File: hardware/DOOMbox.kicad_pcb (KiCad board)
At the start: 4 copper layers, 84 parts, among them J1 DE15_Socket_HighDensity, J2 AudioJack3, SW1 SW_SPST, SW2 SW_Push, U1 RPi Pico 2, U3 AP7381-50SA-7, U4 LM324N, U5 CD4010BE

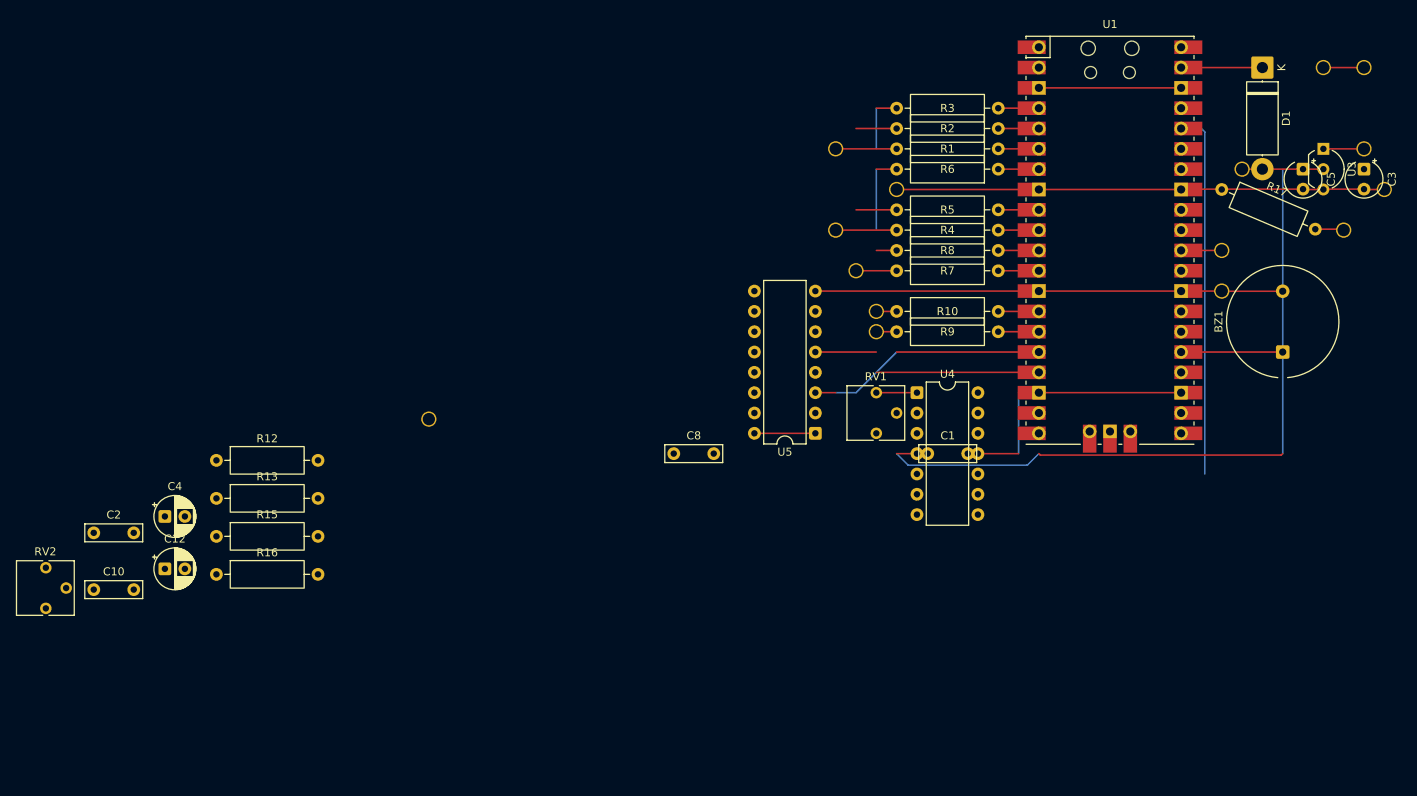
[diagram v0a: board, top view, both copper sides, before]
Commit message: Complete stripboard design
Squashed commit of the following:

commit dbad1e7bdfb2dba54c7140f3a2191c6905e5781a
Author: Jack Bennett <jackbennett0708@gmail.com>
Date:   Sat Aug 30 16:36:03 2025 +0100

    Complete

commit 05059f46a42e6744a15d06e69ba94dfb8af3ae9c
Author: Jack Bennett <jackbennett0708@gmail.com>
Date:   Sat Aug 30 14:41:32 2025 +0100

    1
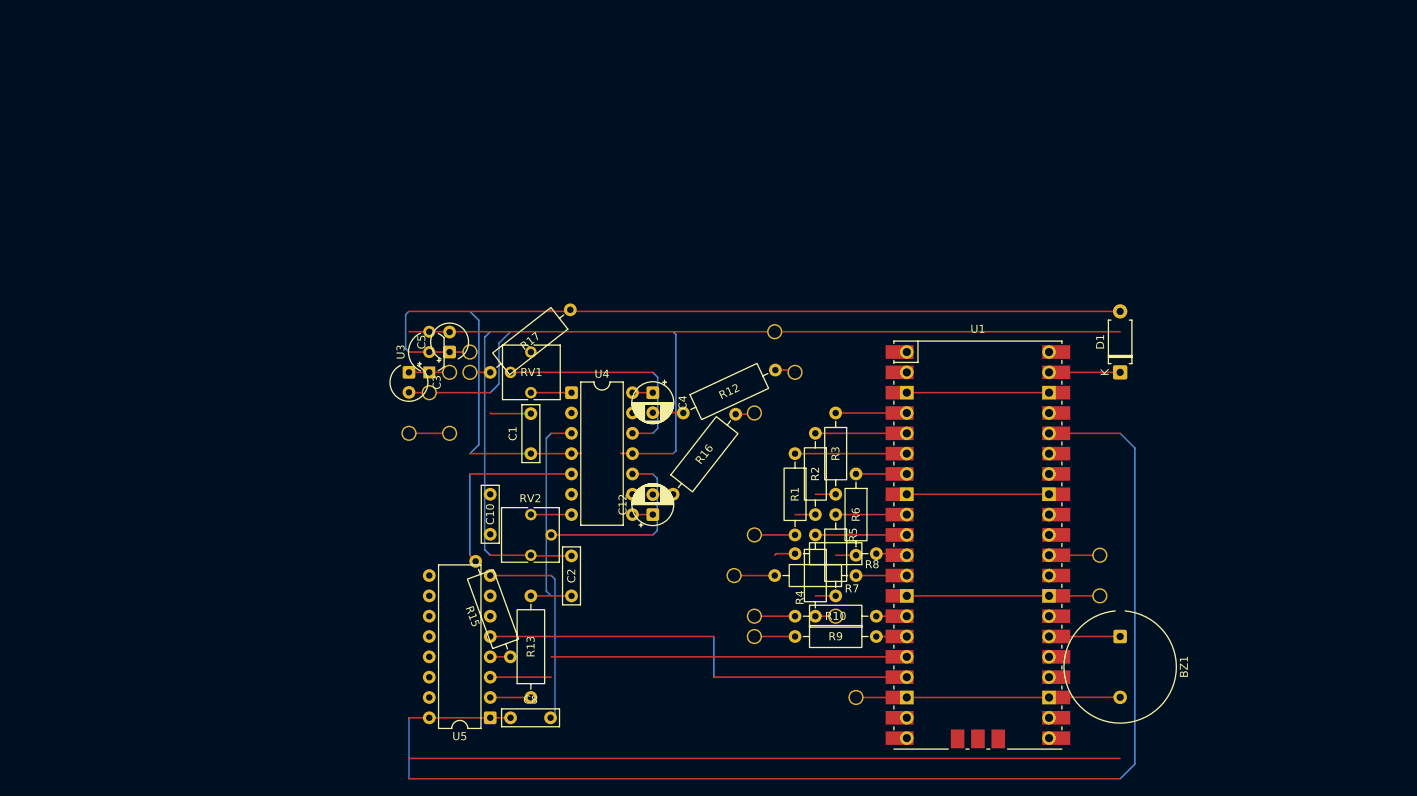
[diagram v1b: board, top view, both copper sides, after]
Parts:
- removed the D2 at (198.1, 48.3)
- removed the D2 at (185.4, 40.6)
- removed the J1 at (139.7, 61.0)
- removed the J1 at (134.6, 48.3)
- removed the J1 at (134.6, 38.1)
- removed the J1 at (142.2, 43.2)
- removed the J1 at (139.7, 58.4)
- removed the J1 at (137.2, 53.3)
- removed the J2 at (83.8, 71.9)
- removed the REF** at (152.4, 40.6)
- removed the REF** at (170.2, 71.1)
- removed the REF** at (141.1, 63.5)
- removed the REF** at (153.8, 71.1)
- removed the REF** at (175.3, 40.6)
- removed the REF** at (175.3, 28.0)
- removed the REF** at (175.3, 50.8)
- removed the REF** at (167.6, 71.1)
- removed the REF** at (193.0, 27.9)
- removed the REF** at (182.9, 40.6)
- removed the REF** at (175.3, 33.0)
- removed the REF** at (152.4, 35.6)
- removed the REF** at (175.3, 35.6)
- removed the REF** at (175.3, 73.7)
- removed the REF** at (198.1, 40.6)
- removed the REF** at (175.3, 63.5)
- removed the REF** at (152.4, 33.0)
- removed the REF** at (203.2, 43.2)
- removed the REF** at (180.3, 25.4)
- removed the REF** at (175.3, 25.4)
- removed the REF** at (175.3, 66.0)
- removed the REF** at (193.0, 48.3)
- removed the REF** at (175.3, 53.3)
- removed the REF** at (175.3, 61.0)
- removed the REF** at (152.4, 50.8)
- removed the REF** at (152.4, 58.4)
- removed the REF** at (175.3, 58.4)
- removed the REF** at (175.3, 38.1)
- removed the REF** at (152.4, 53.3)
- removed the REF** at (175.3, 45.7)
- removed the REF** at (152.4, 48.3)
- removed the REF** at (152.4, 61.0)
- removed the REF** at (180.3, 33.0)
- removed the REF** at (152.4, 45.7)
- removed the REF** at (193.0, 38.1)
- removed the REF** at (175.3, 48.3)
- removed the REF** at (148.6, 76.2)
- removed the REF** at (152.4, 38.1)
- removed the REF** at (175.3, 71.1)
- removed the REF** at (200.7, 27.9)
- removed the SW1 at (200.7, 38.1)
- removed the SW1 at (195.6, 27.9)
- removed the SW2 at (182.9, 50.8)
- removed the SW2 at (182.9, 55.9)
- added ?: , , F.Cu at (124.5, 96.5)
- added ?: , , F.Cu at (134.6, 96.5)
- added ?: , , F.Cu at (124.5, 99.1)
- added ?: , , F.Cu at (137.2, 106.7)
- added ?: , , F.Cu at (121.9, 91.4)
- added D2: LED, Stripboard:Peripheral_Offboard, F.Cu at (88.9, 66.0)
- added J1: DE15_Socket_HighDensity, Stripboard:Peripheral_Offboard, F.Cu at (124.5, 86.4)
- added J2: AudioJack3, Stripboard:Peripheral_Offboard, F.Cu at (127.0, 61.0)
- added J2: AudioJack3, Stripboard:Peripheral_Offboard, F.Cu at (124.5, 71.1)
- added J2: AudioJack3, Stripboard:Peripheral_Offboard, F.Cu at (129.5, 66.0)
- added REF**: Peripheral_Offboard, Stripboard:Peripheral_Offboard, F.Cu at (88.9, 63.5)
- added REF**: Stripboard_Cut, Stripboard:Stripboard_Cut, F.Cu at (126.1, 88.9)
- added REF**: Stripboard_Cut, Stripboard:Stripboard_Cut, F.Cu at (104.1, 83.8)
- added REF**: Stripboard_Cut, Stripboard:Stripboard_Cut, F.Cu at (121.9, 99.1)
- added REF**: Stripboard_Cut, Stripboard:Stripboard_Cut, F.Cu at (154.9, 76.2)
- added REF**: Stripboard_Cut, Stripboard:Stripboard_Cut, F.Cu at (154.9, 99.1)
- added REF**: Stripboard_Cut, Stripboard:Stripboard_Cut, F.Cu at (138.0, 99.0)
- added REF**: Stripboard_Cut, Stripboard:Stripboard_Cut, F.Cu at (154.9, 104.1)
- added REF**: Peripheral_Offboard, Stripboard:Peripheral_Offboard, F.Cu at (81.3, 73.7)
- added REF**: Stripboard_Cut, Stripboard:Stripboard_Cut, F.Cu at (114.3, 83.8)
- added REF**: Stripboard_Cut, Stripboard:Stripboard_Cut, F.Cu at (154.9, 86.4)
- added REF**: Stripboard_Cut, Stripboard:Stripboard_Cut, F.Cu at (131.1, 81.3)
- added REF**: Stripboard_Cut, Stripboard:Stripboard_Cut, F.Cu at (114.3, 68.6)
- added REF**: Stripboard_Cut, Stripboard:Stripboard_Cut, F.Cu at (133.4, 83.8)
- added REF**: Stripboard_Cut, Stripboard:Stripboard_Cut, F.Cu at (104.1, 78.7)
- added REF**: Stripboard_Cut, Stripboard:Stripboard_Cut, F.Cu at (154.9, 109.2)
- added REF**: Stripboard_Cut, Stripboard:Stripboard_Cut, F.Cu at (154.9, 71.1)
- added REF**: Stripboard_Cut, Stripboard:Stripboard_Cut, F.Cu at (110.5, 71.1)
- added REF**: Stripboard_Cut, Stripboard:Stripboard_Cut, F.Cu at (116.8, 81.3)
- added REF**: Stripboard_Cut, Stripboard:Stripboard_Cut, F.Cu at (87.6, 91.4)
- added REF**: Stripboard_Cut, Stripboard:Stripboard_Cut, F.Cu at (119.4, 91.4)
- added REF**: Stripboard_Cut, Stripboard:Stripboard_Cut, F.Cu at (154.9, 96.5)
- added REF**: Stripboard_Cut, Stripboard:Stripboard_Cut, F.Cu at (93.0, 86.3)
- added REF**: Stripboard_Cut, Stripboard:Stripboard_Cut, F.Cu at (129.5, 94.0)
- added REF**: Stripboard_Cut, Stripboard:Stripboard_Cut, F.Cu at (87.6, 106.7)
- added REF**: Stripboard_Cut, Stripboard:Stripboard_Cut, F.Cu at (87.6, 101.6)
- added REF**: Stripboard_Cut, Stripboard:Stripboard_Cut, F.Cu at (114.3, 73.7)
- added REF**: Stripboard_Cut, Stripboard:Stripboard_Cut, F.Cu at (130.7, 86.4)
- added REF**: Stripboard_Cut, Stripboard:Stripboard_Cut, F.Cu at (121.9, 86.4)
- added REF**: Stripboard_Cut, Stripboard:Stripboard_Cut, F.Cu at (133.5, 88.9)
- added REF**: Stripboard_Cut, Stripboard:Stripboard_Cut, F.Cu at (94.0, 63.5)
- added REF**: Stripboard_Cut, Stripboard:Stripboard_Cut, F.Cu at (92.9, 66.1)
- added REF**: Stripboard_Cut, Stripboard:Stripboard_Cut, F.Cu at (110.8, 81.3)
- added REF**: Stripboard_Cut, Stripboard:Stripboard_Cut, F.Cu at (132.1, 91.4)
- added REF**: Stripboard_Cut, Stripboard:Stripboard_Cut, F.Cu at (114.3, 78.7)
- added REF**: Stripboard_Cut, Stripboard:Stripboard_Cut, F.Cu at (154.9, 63.5)
- added REF**: Stripboard_Cut, Stripboard:Stripboard_Cut, F.Cu at (87.6, 94.0)
- added REF**: Stripboard_Cut, Stripboard:Stripboard_Cut, F.Cu at (132.1, 66.0)
- added REF**: Stripboard_Cut, Stripboard:Stripboard_Cut, F.Cu at (121.9, 96.5)
- added REF**: Stripboard_Cut, Stripboard:Stripboard_Cut, F.Cu at (104.1, 71.1)
- added REF**: Stripboard_Cut, Stripboard:Stripboard_Cut, F.Cu at (116.8, 71.1)
- added REF**: Stripboard_Cut, Stripboard:Stripboard_Cut, F.Cu at (149.9, 63.5)
- added REF**: Stripboard_Cut, Stripboard:Stripboard_Cut, F.Cu at (138.0, 96.5)
- added REF**: Stripboard_Cut, Stripboard:Stripboard_Cut, F.Cu at (88.9, 73.7)
- added REF**: Stripboard_Cut, Stripboard:Stripboard_Cut, F.Cu at (87.6, 96.5)
- added REF**: Stripboard_Cut, Stripboard:Stripboard_Cut, F.Cu at (137.2, 94.0)
- added REF**: Stripboard_Cut, Stripboard:Stripboard_Cut, F.Cu at (87.6, 99.1)
- added REF**: Stripboard_Cut, Stripboard:Stripboard_Cut, F.Cu at (154.9, 88.9)
- added REF**: Stripboard_Cut, Stripboard:Stripboard_Cut, F.Cu at (116.8, 76.2)
- added REF**: Stripboard_Cut, Stripboard:Stripboard_Cut, F.Cu at (101.6, 104.1)
- added REF**: Stripboard_Cut, Stripboard:Stripboard_Cut, F.Cu at (128.4, 83.9)
- added REF**: Stripboard_Cut, Stripboard:Stripboard_Cut, F.Cu at (154.9, 101.6)
- added REF**: Stripboard_Cut, Stripboard:Stripboard_Cut, F.Cu at (100.0, 71.0)
- added REF**: Stripboard_Cut, Stripboard:Stripboard_Cut, F.Cu at (136.2, 78.7)
- added REF**: Stripboard_Cut, Stripboard:Stripboard_Cut, F.Cu at (154.9, 91.4)
- added REF**: Stripboard_Cut, Stripboard:Stripboard_Cut, F.Cu at (101.6, 109.2)
- added REF**: Stripboard_Cut, Stripboard:Stripboard_Cut, F.Cu at (99.1, 63.5)
- added REF**: Peripheral_Offboard, Stripboard:Peripheral_Offboard, F.Cu at (86.4, 66.0)
- added REF**: Stripboard_Cut, Stripboard:Stripboard_Cut, F.Cu at (130.9, 96.5)
- added REF**: Stripboard_Cut, Stripboard:Stripboard_Cut, F.Cu at (104.1, 68.6)
- added REF**: Stripboard_Cut, Stripboard:Stripboard_Cut, F.Cu at (92.7, 96.5)
- added REF**: Stripboard_Cut, Stripboard:Stripboard_Cut, F.Cu at (130.6, 73.6)
- added REF**: Stripboard_Cut, Stripboard:Stripboard_Cut, F.Cu at (101.6, 106.7)
- added REF**: Stripboard_Cut, Stripboard:Stripboard_Cut, F.Cu at (154.9, 66.0)
- added REF**: Stripboard_Cut, Stripboard:Stripboard_Cut, F.Cu at (87.6, 104.1)
- added REF**: Stripboard_Cut, Stripboard:Stripboard_Cut, F.Cu at (157.5, 111.8)
- added REF**: Stripboard_Cut, Stripboard:Stripboard_Cut, F.Cu at (87.4, 66.1)
- added REF**: Stripboard_Cut, Stripboard:Stripboard_Cut, F.Cu at (104.1, 76.2)
- added REF**: Peripheral_Offboard, Stripboard:Peripheral_Offboard, F.Cu at (167.6, 94.0)
- added REF**: Stripboard_Cut, Stripboard:Stripboard_Cut, F.Cu at (149.9, 66.0)
- added REF**: Stripboard_Cut, Stripboard:Stripboard_Cut, F.Cu at (114.3, 66.0)
- added REF**: Stripboard_Cut, Stripboard:Stripboard_Cut, F.Cu at (154.9, 73.7)
- added REF**: Stripboard_Cut, Stripboard:Stripboard_Cut, F.Cu at (94.0, 68.6)
- added REF**: Stripboard_Cut, Stripboard:Stripboard_Cut, F.Cu at (100.2, 81.3)
- added REF**: Stripboard_Cut, Stripboard:Stripboard_Cut, F.Cu at (133.3, 71.1)
- added REF**: Stripboard_Cut, Stripboard:Stripboard_Cut, F.Cu at (92.5, 94.0)
- added REF**: Stripboard_Cut, Stripboard:Stripboard_Cut, F.Cu at (90.3, 89.0)
- added REF**: Peripheral_Offboard, Stripboard:Peripheral_Offboard, F.Cu at (83.8, 68.6)
- added REF**: Stripboard_Cut, Stripboard:Stripboard_Cut, F.Cu at (104.1, 73.7)
- added REF**: Stripboard_Cut, Stripboard:Stripboard_Cut, F.Cu at (84.9, 111.8)
- added REF**: Stripboard_Cut, Stripboard:Stripboard_Cut, F.Cu at (135.8, 91.5)
- added REF**: Stripboard_Cut, Stripboard:Stripboard_Cut, F.Cu at (154.9, 83.8)
- added REF**: Stripboard_Cut, Stripboard:Stripboard_Cut, F.Cu at (138.7, 88.7)
- added REF**: Stripboard_Cut, Stripboard:Stripboard_Cut, F.Cu at (154.9, 78.7)
- added REF**: Stripboard_Cut, Stripboard:Stripboard_Cut, F.Cu at (104.1, 81.3)
- added REF**: Stripboard_Cut, Stripboard:Stripboard_Cut, F.Cu at (128.3, 76.2)
- added SW1: SW_SPST, Stripboard:Peripheral_Offboard, F.Cu at (86.4, 73.7)
- added SW2: SW_Push, Stripboard:Peripheral_Offboard, F.Cu at (167.6, 88.9)
- D1: footprint Diode_THT:D_5W_P12.70mm_Horizontal -> Diode_THT:D_A-405_P7.62mm_Horizontal
- R1, R10, R2, R3, R4, R5, R6, R7, R8, R9: footprint Resistor_THT:R_Axial_DIN0309_L9.0mm_D3.2mm_P12.70mm_Horizontal -> Resistor_THT:R_Axial_DIN0207_L6.3mm_D2.5mm_P10.16mm_Horizontal
- moved C3 122.1 mm to (81.3, 66.0)
- moved U3 115.2 mm to (83.8, 66.0), turned to 90 degrees
- moved C5 109.1 mm to (86.4, 63.5), turned to 90 degrees
- moved R17 82.8 mm to (101.4, 58.2), turned to -142 degrees
- moved C4 62.9 mm to (111.8, 68.6), turned to -90 degrees
- moved C12 61.4 mm to (111.8, 83.8), turned to 90 degrees
- moved RV2 61.0 mm to (96.5, 88.9)
- moved C2 60.2 mm to (101.6, 94.0), turned to 90 degrees
- moved R12 58.7 mm to (115.6, 71.1), turned to 25 degrees
- moved R16 58.0 mm to (114.3, 81.3), turned to 52 degrees
- moved U5 54.0 mm to (91.4, 109.2)
- moved C10 51.0 mm to (91.4, 81.3), turned to -90 degrees
- moved C1 49.6 mm to (96.5, 76.2), turned to 90 degrees
- moved R13 46.5 mm to (96.5, 106.7), turned to 90 degrees
- moved R1 45.8 mm to (129.5, 76.2), turned to -90 degrees
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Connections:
- C12 pad 2: Net-(C12-Pad2) -> (no net)
- C4 pad 2: Net-(C4-Pad2) -> (no net)
- C8 pad 1: (no net) -> +3V3
- C8 pad 2: (no net) -> GND
- R12 pad 1: Net-(C4-Pad2) -> (no net)
- R12 pad 2: Net-(J2-PadT) -> (no net)
- R15 pad 2: Net-(U4B-+) -> (no net)
- R16 pad 1: Net-(C12-Pad2) -> (no net)
- RV2 pad 2: Net-(U4C-+) -> (no net)
- U1 pad 25: Net-(BZ1-+) -> unconnected-(U1-GPIO19-Pad25)
- U1 pad 26: unconnected-(U1-GPIO20-Pad26) -> Net-(BZ1-+)
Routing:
- net GND: track 176.9 -> 484.8 mm
- net +3V3: track 7.62 -> 110.5 mm
- net PWM_AUL: track 20.3 -> 52.1 mm
- net Net-(U4D--): track 2.54 -> 32.6 mm
- net +5V: track 49.6 -> 21.5 mm
- net PWM_AUR: track 30.5 -> 52.1 mm
- net Net-(D2-K): track 3.60 -> 21.2 mm
- net Net-(U4B-+): track 0.00 -> 15.2 mm
- net Net-(U4C--): track 2.54 -> 15.7 mm
- net VGA_R2: track 5.08 -> 14.0 mm
- net unconnected-(U5-D-Pad9): track 7.62 -> 0.00 mm
- net Net-(U4A-+): track 0.00 -> 7.62 mm
- net VGA_R1: track 5.08 -> 11.4 mm
- net VGA_G2: track 5.08 -> 11.4 mm
- net Net-(U5-G): track 0.00 -> 5.08 mm
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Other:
- board text added: "3V3"
- board text added: "5V"
- board text added: "D2"
- board text added: "DOOMbox"
- board text added: "GND"
- board text added: "J2"
- board text added: "R7, R8 on top + horiz"
- board text added: "SW1"
- board text added: "SW2"
